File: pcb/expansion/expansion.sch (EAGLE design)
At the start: 36 parts, among them IC3 STM32F042F4, J1 AUDIO_JACK_3.5MM_PTH, J2 AUDIO_JACK_3.5MM_PTH, J3 AUDIO_JACK_3.5MM_PTH, J4 AUDIO_JACK_3.5MM_PTH, J5 AUDIO_JACK_3.5MM_PTH, J6 AUDIO_JACK_3.5MM_PTH, SW3 324_SW, SW4 324_SW, U1 USBC_16P, U2 USBC_16P, U4 XC6206_DEV

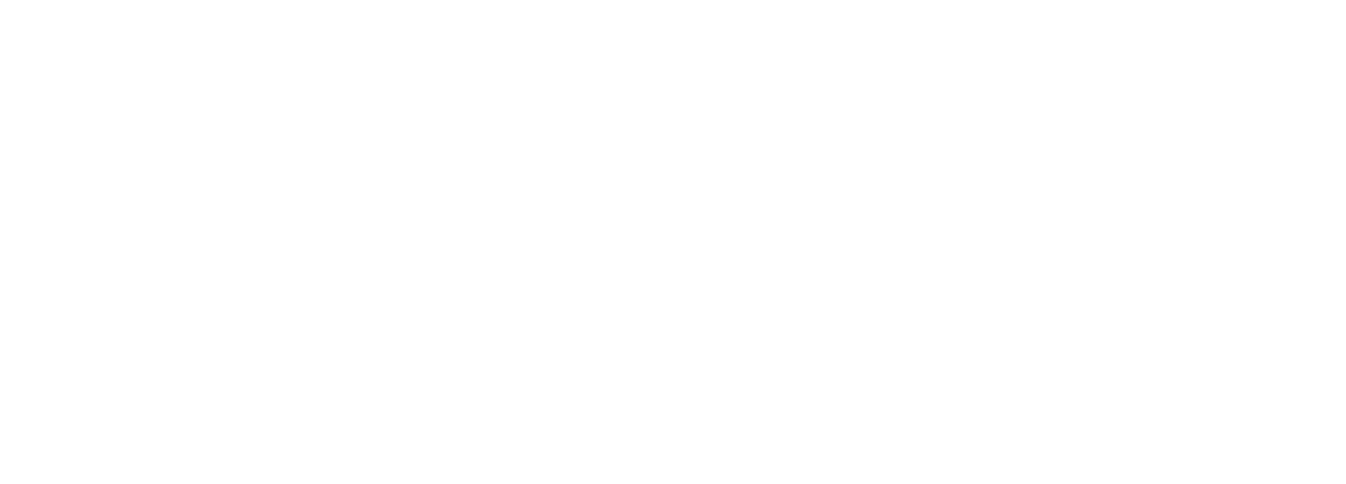
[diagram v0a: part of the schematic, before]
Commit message: working on pcb
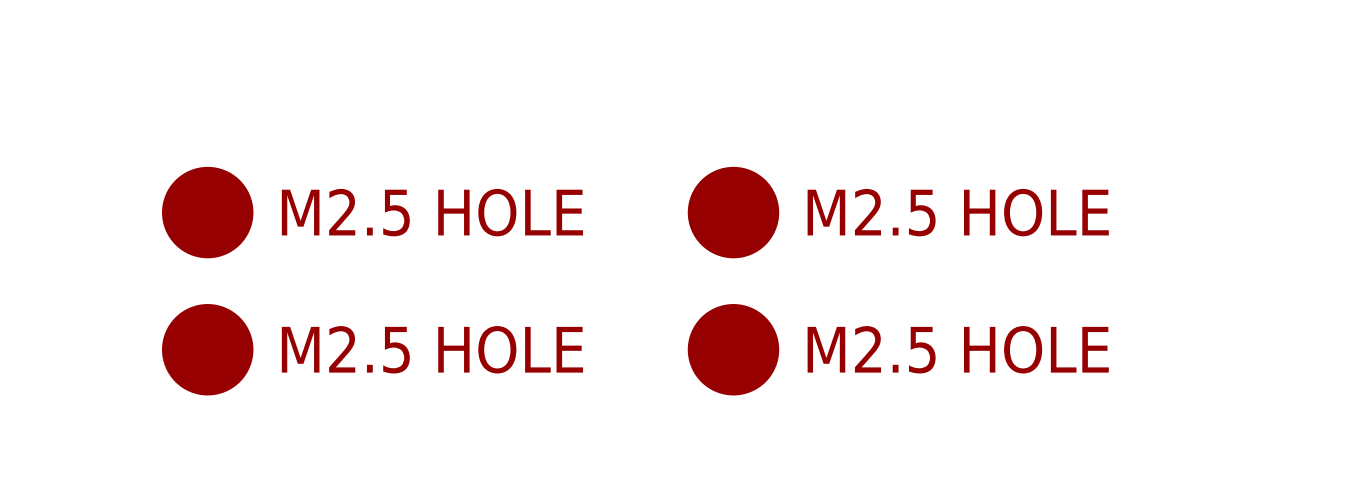
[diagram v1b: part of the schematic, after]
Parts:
- added U$10, U$11, U$8, U$9: M2.5HOLE, f1c100s:M2.5HOLE
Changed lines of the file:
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@@
 <part name="JP5" library="pinhead" library_urn="urn:adsk.eagle:library:325" deviceset="PINHD-1X3" device="" package3d_urn="urn:adsk.eagle:package:22458/2"/>
 <part name="JP6" library="pinhead" library_urn="urn:adsk.eagle:library:325" deviceset="PINHD-1X3" device="" package3d_urn="urn:adsk.eagle:package:22458/2"/>
+<part name="U$8" library="f1c100s" deviceset="M2.5HOLE" device=""/>
+<part name="U$9" library="f1c100s" deviceset="M2.5HOLE" device=""/>
+<part name="U$10" library="f1c100s" deviceset="M2.5HOLE" device=""/>
+<part name="U$11" library="f1c100s" deviceset="M2.5HOLE" device=""/>
 </parts>
 <sheets>
@@
 <attribute name="VALUE" x="168.91" y="-101.6" size="1.778" layer="96"/>
 </instance>
+<instance part="U$8" gate="G$1" x="238.76" y="-71.12" smashed="yes"/>
+<instance part="U$9" gate="G$1" x="238.76" y="-86.36" smashed="yes"/>
+<instance part="U$10" gate="G$1" x="297.18" y="-71.12" smashed="yes"/>
+<instance part="U$11" gate="G$1" x="297.18" y="-86.36" smashed="yes"/>
 </instances>
 <busses>
